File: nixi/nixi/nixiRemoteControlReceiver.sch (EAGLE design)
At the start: 16 parts, among them IC1 7805L, IC2 4081D, IC3 40106D, K1 TXD2-1.5V, K2 TXD2-1.5V, T1 2N3904, T2 2N3904

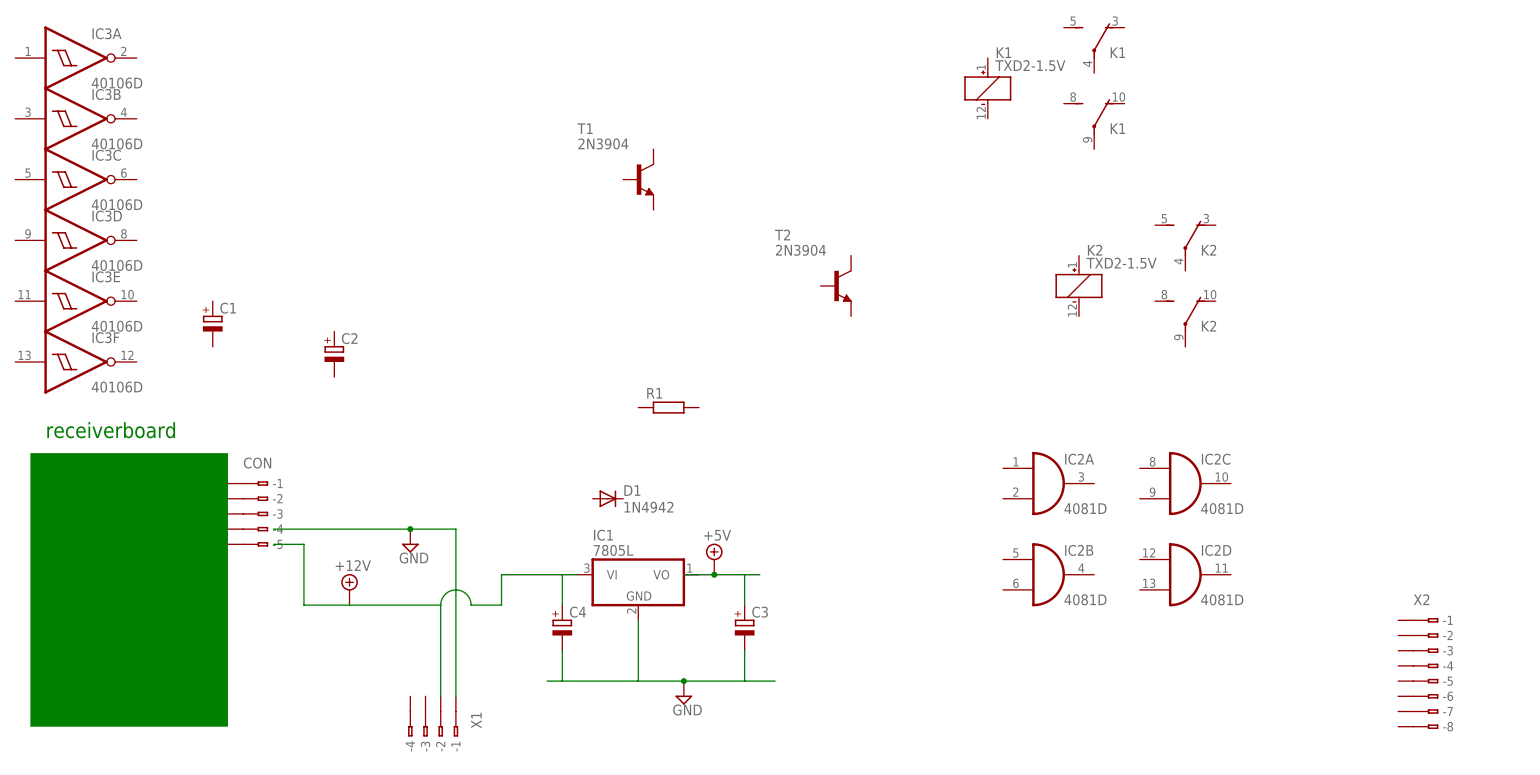
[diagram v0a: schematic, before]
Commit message: nixi started
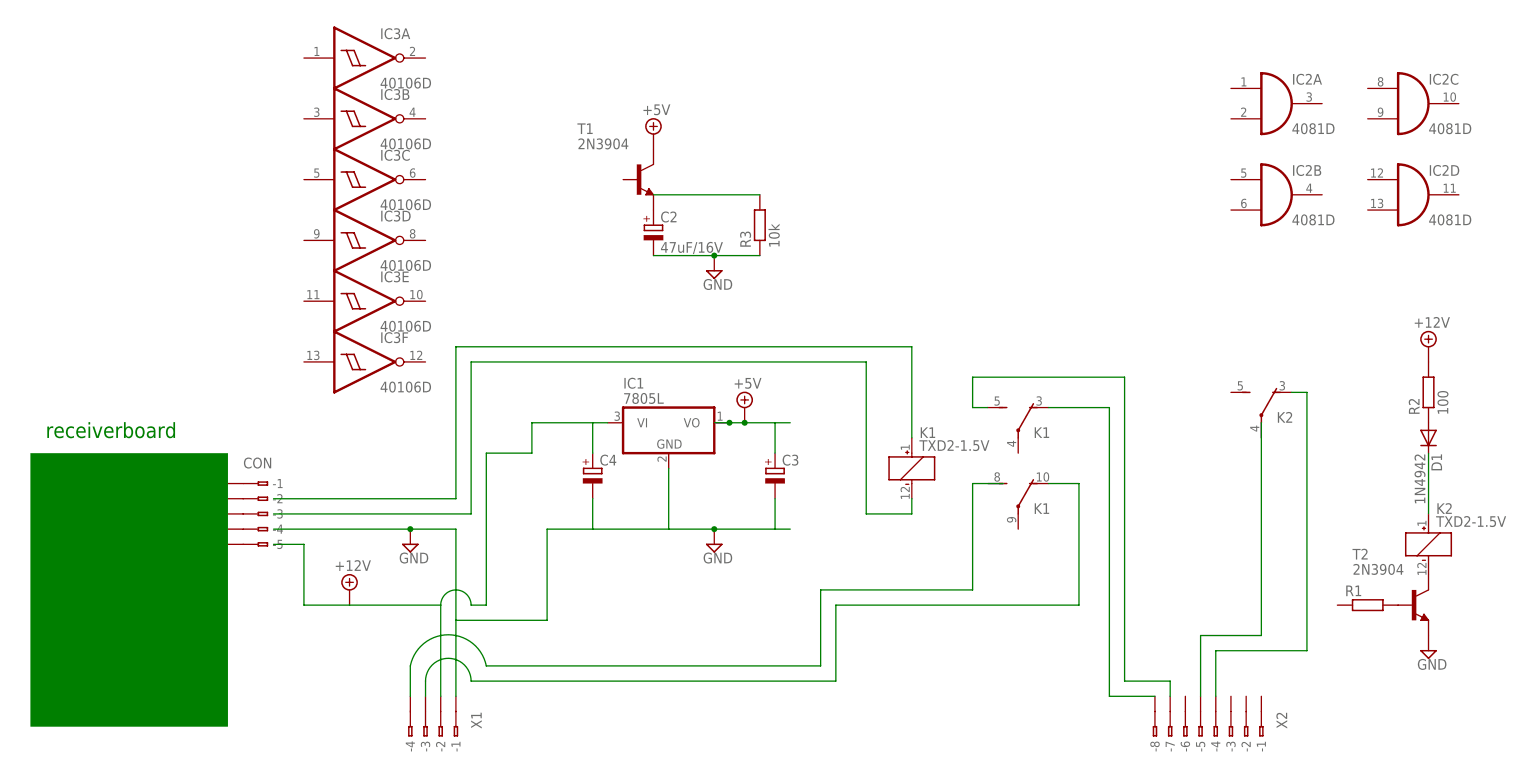
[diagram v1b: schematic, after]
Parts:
- removed C1: (no value), resistor:CPOL-EUE10-20
- added R2: 100, resistor:R-EU_0411/15
- added R3: 10k, resistor:R-EU_0411/15
- C2: value (none) -> 47uF/16V
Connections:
- new net N$1: K1G$2.O, X1.B-3
- new net N$10: D1.C, K2_.+
- new net N$11: C2.+, T1.E
- new net N$12: R3.2
- new net N$13: K1_.-
- new net N$14: K1_.+
- new net N$2: X1.B-4
- new net N$3: K1G$1.O, X2.B-8
- new net N$4: K1G$1.S, X2.B-7
- new net N$5: K2_.-, T2.C
- new net N$6: R1.2, T2.B
- new net N$7: K2G$1.O, X2.B-4
- new net N$8: X2.B-5
- new net N$9: D1.A, R2.1
- net +12V: now also R2.2
- net +5V: now also IC1.VO, T1.C
- net GND: now also C2.-, R3.1, T2.E
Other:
- moved on the sheet: C2, C3, C4, D1, IC1, IC2A, IC2B, IC2C, IC2D, IC3A, IC3B, IC3C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
